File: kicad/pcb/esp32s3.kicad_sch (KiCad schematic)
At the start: 16 parts, among them J1 ESP JTAG, J3 ESP UART, SW1 ESP Boot, SW2 ESP Rst, U3 ESP32-S3-WROOM-2, Y2 32.768 KHz

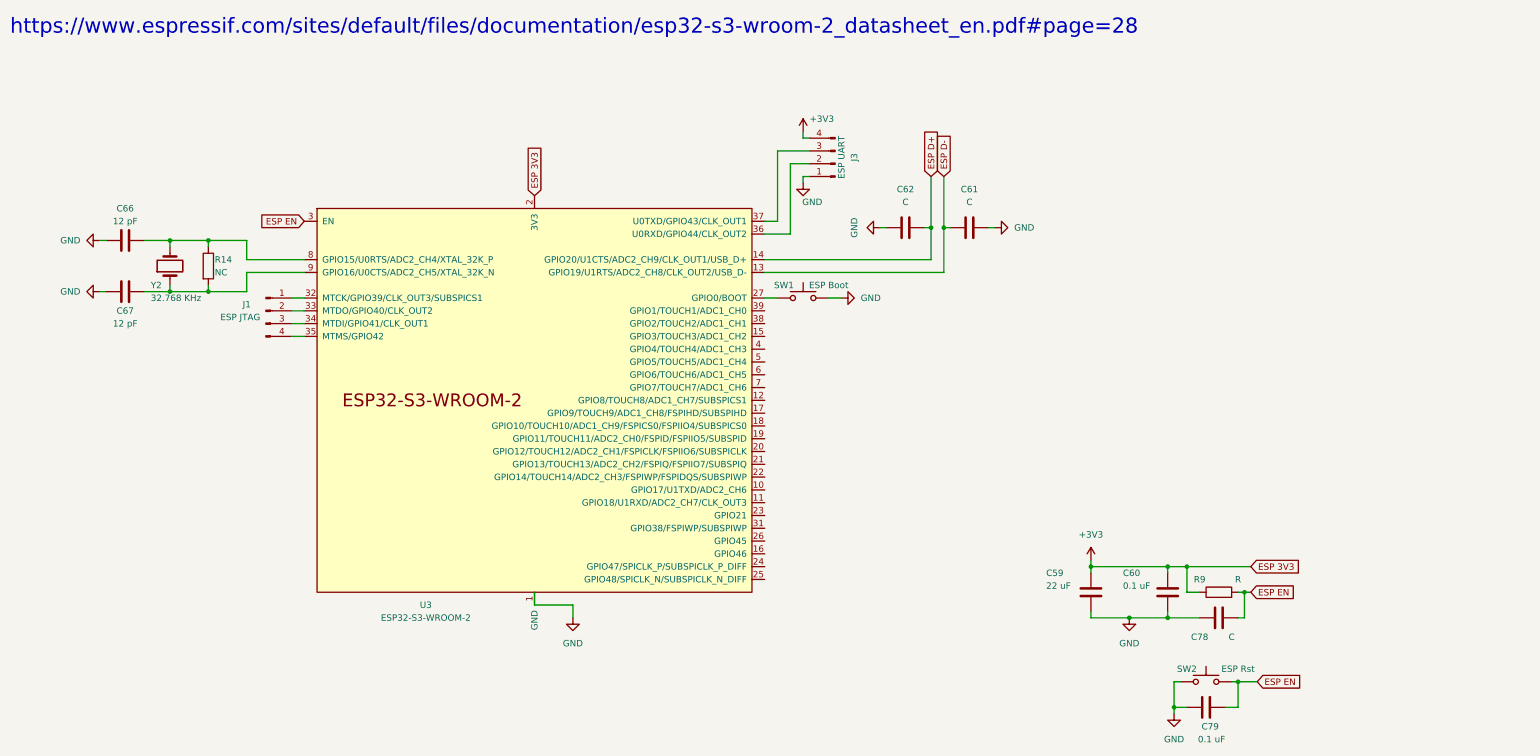
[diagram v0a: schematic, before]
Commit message: Initial wiring sorted out?
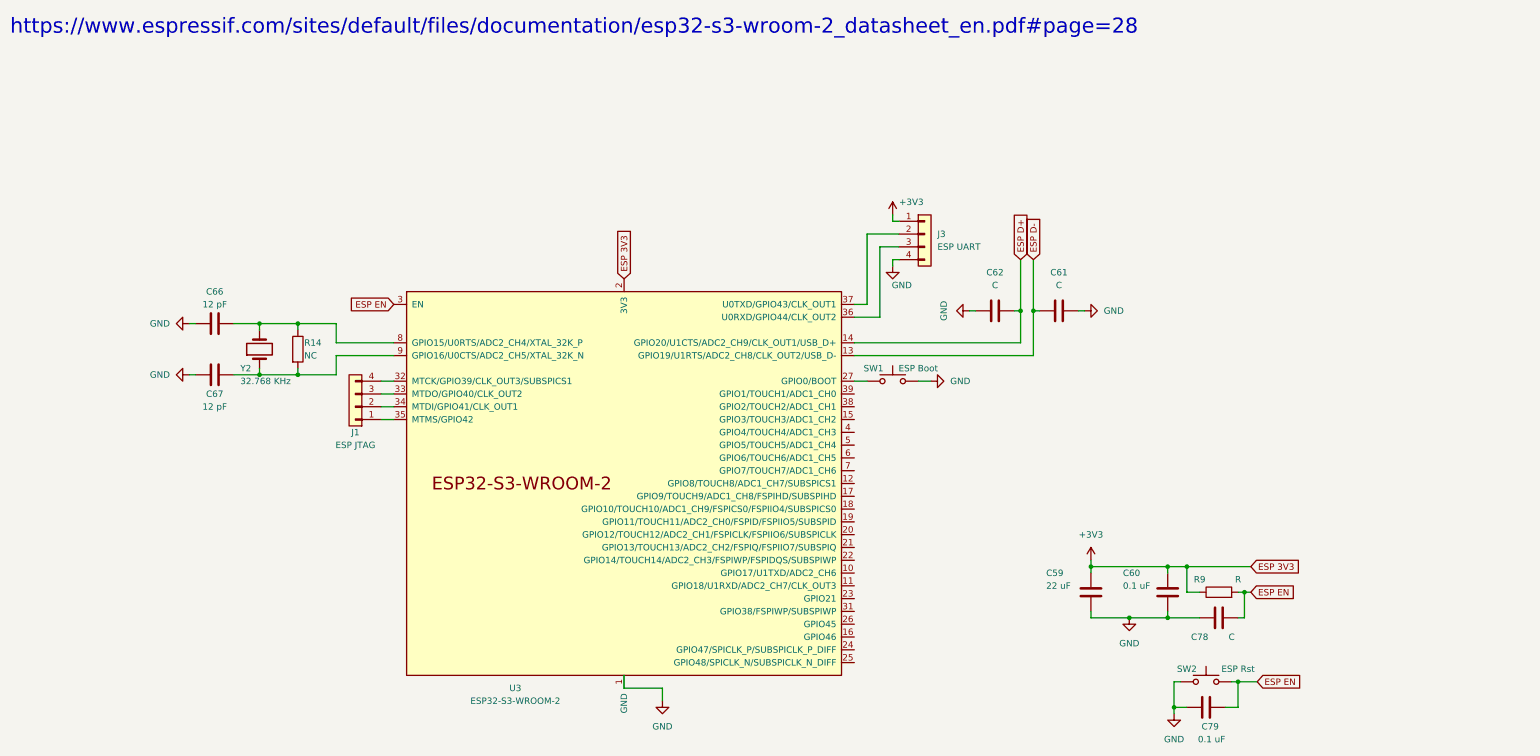
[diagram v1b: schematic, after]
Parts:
- removed J1: ESP JTAG, symbol Connector:Conn_01x04_Pin
- removed J3: ESP UART, symbol Connector:Conn_01x04_Pin
- added J1: ESP JTAG, symbol Connector_Generic:Conn_01x04
- added J3: ESP UART, symbol Connector_Generic:Conn_01x04
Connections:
- net +3V3: now also J3.1 (Pin_1)
- net GND: now also J3.4 (Pin_4)
- net at U3.36 (U0RXD/GPIO44/CLK_OUT2): now also J3.3 (Pin_3)
- net at U3.37 (U0TXD/GPIO43/CLK_OUT1): now also J3.2 (Pin_2)
- net at U3.32 (MTCK/GPIO39/CLK_OUT3/SUBSPICS1): now also J1.4 (Pin_4)
- net at U3.33 (MTDO/GPIO40/CLK_OUT2): now also J1.3 (Pin_3)
- net at U3.34 (MTDI/GPIO41/CLK_OUT1): now also J1.2 (Pin_2)
- net at U3.35 (MTMS/GPIO42): now also J1.1 (Pin_1)
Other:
- moved on the sheet: C61, C62, C66, C67, R14, SW1, U3, Y2
